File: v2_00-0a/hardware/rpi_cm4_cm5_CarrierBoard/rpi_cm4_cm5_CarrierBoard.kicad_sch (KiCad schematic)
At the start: 0 parts

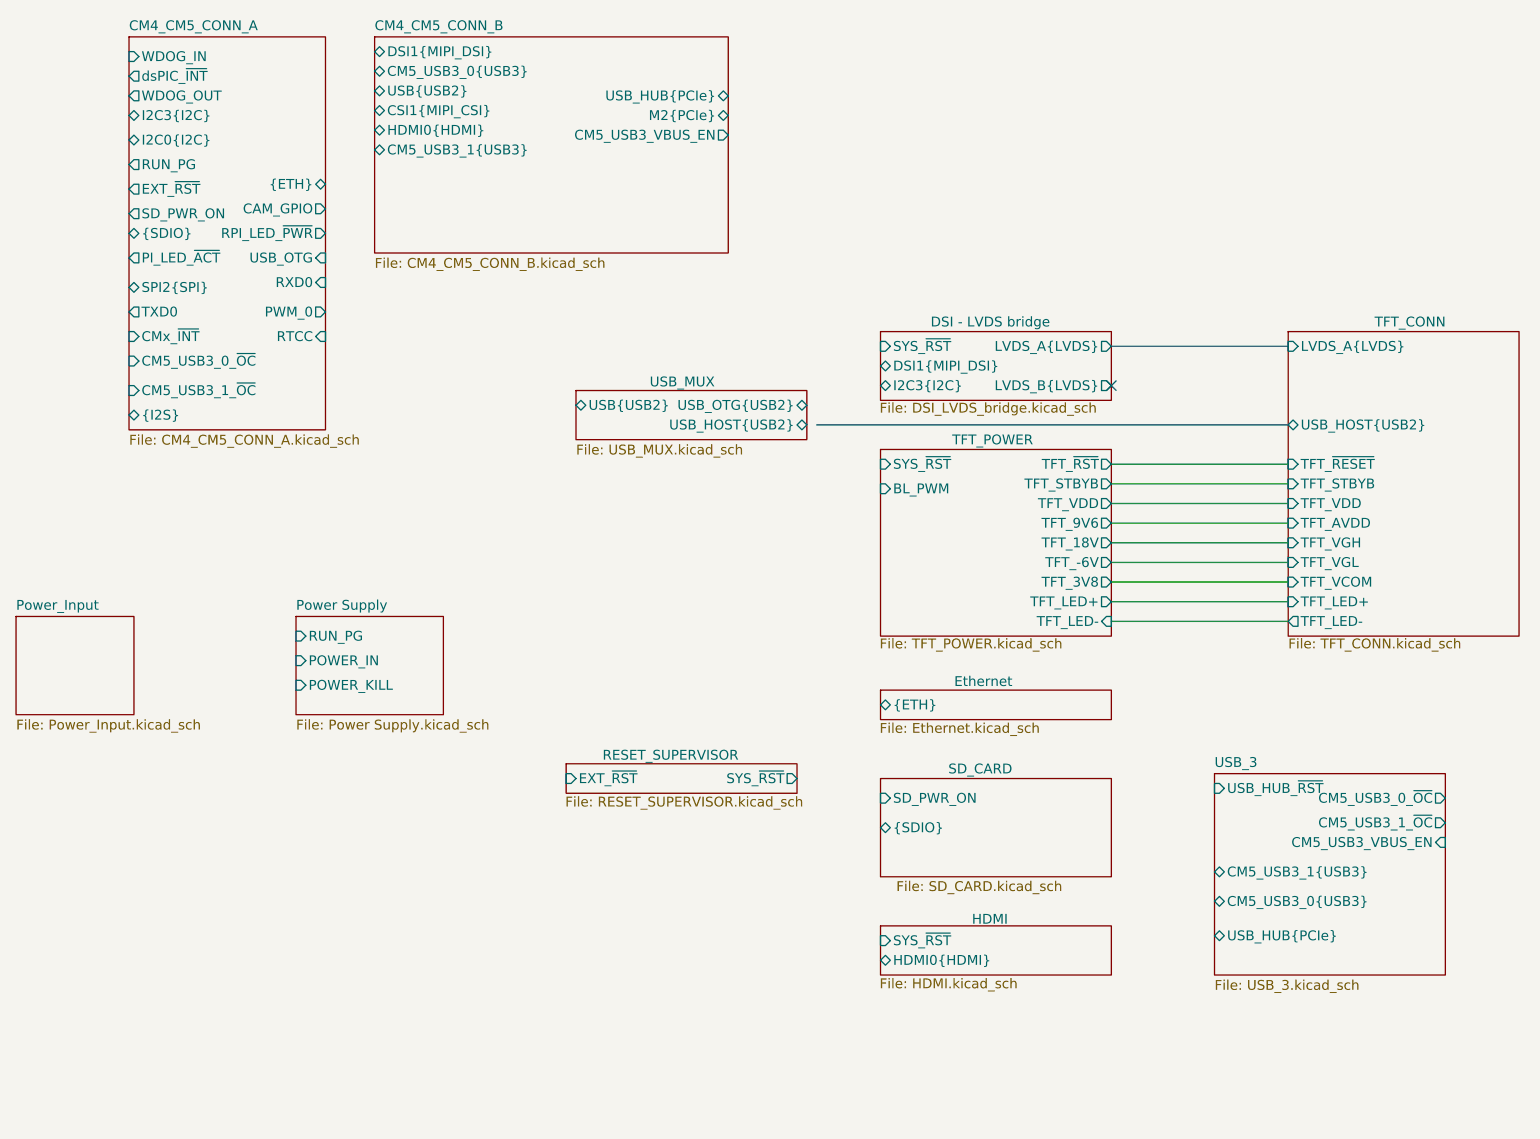
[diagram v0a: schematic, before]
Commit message: Add and modify existing schematics
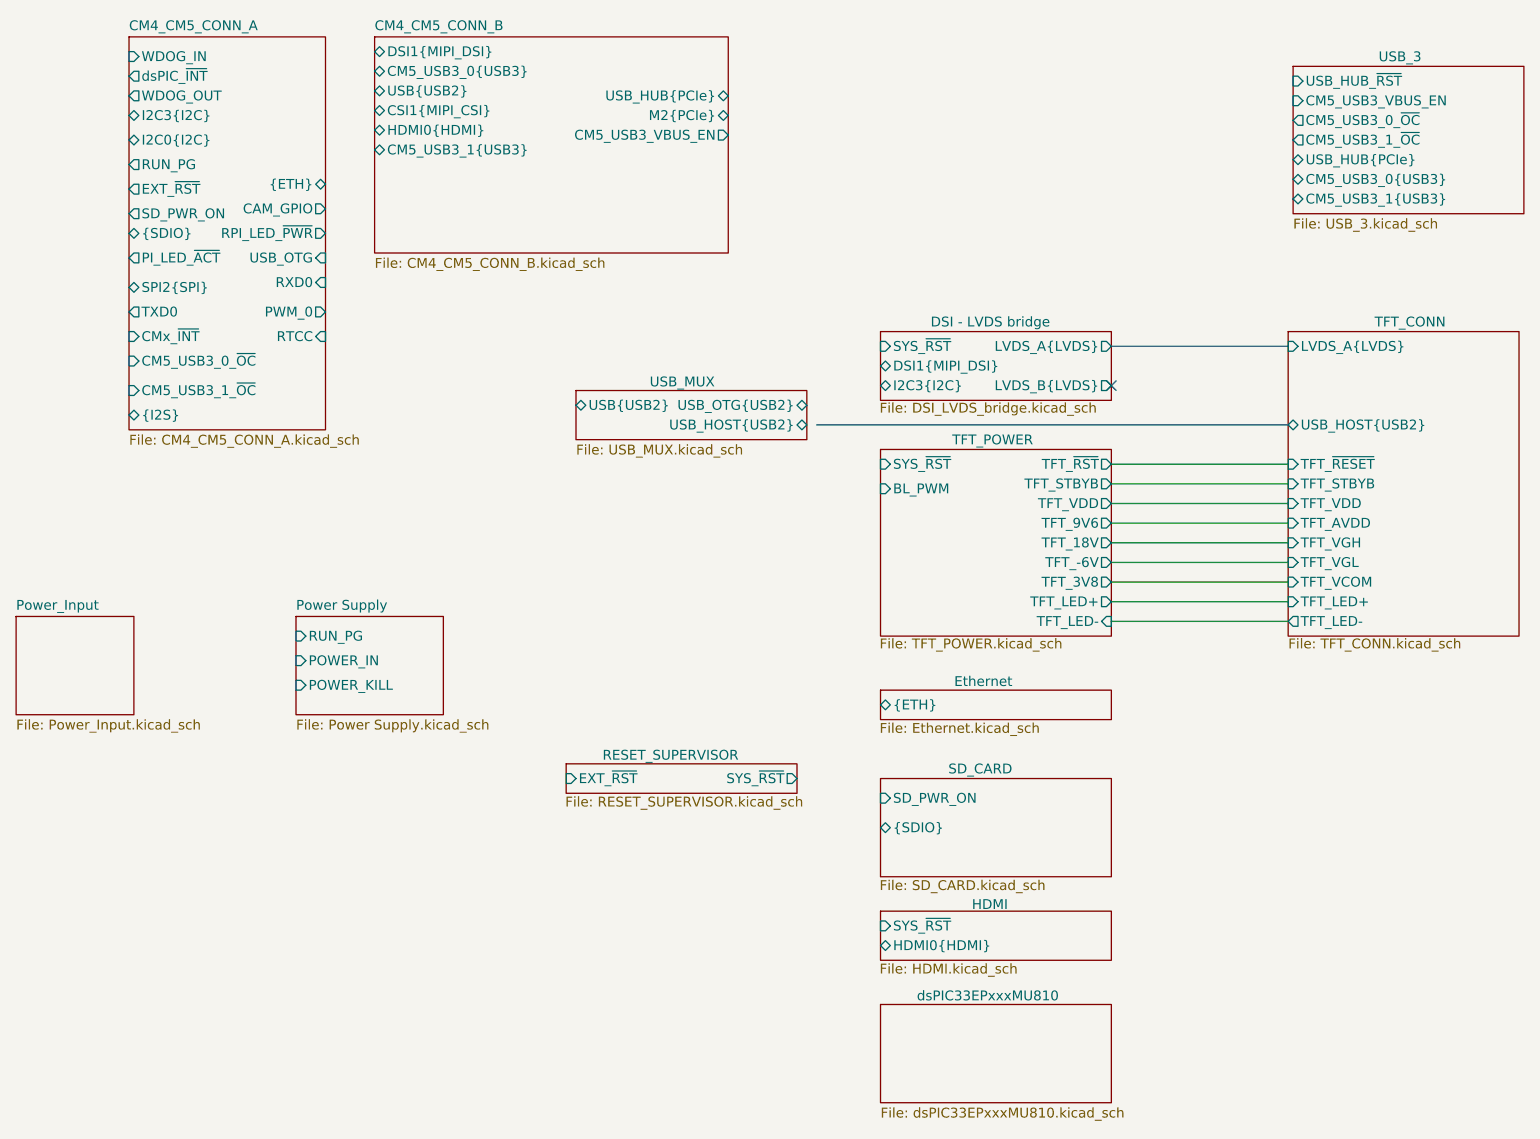
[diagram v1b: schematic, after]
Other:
- added sheet dsPIC33EPxxxMU810 (dsPIC33EPxxxMU810.kicad_sch)
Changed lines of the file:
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@@
 	)
 	(sheet
-		(at 241.935 120.65)
-		(size 29.845 26.035)
+		(at 252.095 29.21)
+		(size 29.845 19.05)
 		(exclude_from_sim no)
 		(in_bom yes)
 		(on_board yes)
 		(dnp no)
-		(fields_autoplaced yes)
 		(stroke
 			(width 0.1524)
@@
 		)
 		(property "Sheetname" "USB_3"
-			(at 241.935 119.9384 0)
+			(at 263.144 28.702 0)
 			(effects
 				(font
@@
 		)
 		(property "Sheetfile" "USB_3.kicad_sch"
-			(at 241.935 147.2696 0)
+			(at 252.095 48.8446 0)
 			(effects
 				(font
@@
 		)
 		(pin "USB_HUB_~{RST}" input
-			(at 241.935 122.555 180)
+			(at 252.095 31.115 180)
 			(effects
 				(font
@@
 		)
 		(pin "CM5_USB3_0{USB3}" bidirectional
-			(at 241.935 137.16 180)
+			(at 252.095 43.815 180)
 			(effects
 				(font
@@
 		)
 		(pin "CM5_USB3_1_~{OC}" output
-			(at 271.78 127 0)
-			(effects
-				(font
-					(size 1.27 1.27)
-				)
-				(justify right)
+			(at 252.095 38.735 180)
+			(effects
+				(font
+					(size 1.27 1.27)
+				)
+				(justify left)
 			)
 		)
 		(pin "CM5_USB3_0_~{OC}" output
-			(at 271.78 123.825 0)
-			(effects
-				(font
-					(size 1.27 1.27)
-				)
-				(justify right)
+			(at 252.095 36.195 180)
+			(effects
+				(font
+					(size 1.27 1.27)
+				)
+				(justify left)
 			)
 		)
 		(pin "CM5_USB3_VBUS_EN" input
-			(at 271.78 129.54 0)
-			(effects
-				(font
-					(size 1.27 1.27)
-				)
-				(justify right)
+			(at 252.095 33.655 180)
+			(effects
+				(font
+					(size 1.27 1.27)
+				)
+				(justify left)
 			)
 		)
 		(pin "CM5_USB3_1{USB3}" bidirectional
-			(at 241.935 133.35 180)
+			(at 252.095 46.355 180)
 			(effects
 				(font
@@
 		)
 		(pin "USB_HUB{PCIe}" bidirectional
-			(at 241.935 141.605 180)
+			(at 252.095 41.275 180)
 			(effects
 				(font
@@
 	)
 	(sheet
+		(at 198.755 150.495)
+		(size 29.845 12.7)
+		(exclude_from_sim no)
+		(in_bom yes)
+		(on_board yes)
+		(dnp no)
+		(stroke
+			(width 0.1524)
+			(type solid)
+		)
+		(fill
+			(color 0 0 0 0.0000)
+		)
+		(property "Sheetname" "dsPIC33EPxxxMU810"
+			(at 203.454 150.114 0)
+			(effects
+				(font
+					(size 1.27 1.27)
+				)
+				(justify left bottom)
+			)
+		)
+		(property "Sheetfile" "dsPIC33EPxxxMU810.kicad_sch"
+			(at 198.755 163.7796 0)
+			(effects
+				(font
+					(size 1.27 1.27)
+				)
+				(justify left top)
+			)
+		)
+		(instances
+			(project "rpi_cm4_cm5_CarrierBoard"
+				(path "/7dcdf741-90ca-4333-848c-806f4d64158e"
+					(page "15")
+				)
+			)
+		)
+	)
+	(sheet
 		(at 158.115 119.38)
 		(size 29.845 3.81)
@@
 		)
 		(property "Sheetfile" "SD_CARD.kicad_sch"
-			(at 200.787 134.493 0)
+			(at 198.628 134.366 0)
 			(effects
 				(font
@@
 	)
 	(sheet
-		(at 198.755 140.335)
+		(at 198.755 138.43)
 		(size 29.845 6.35)
 		(exclude_from_sim no)
@@
 		)
 		(property "Sheetname" "HDMI"
-			(at 210.566 140.208 0)
+			(at 210.566 138.303 0)
 			(effects
 				(font
@@
 		)
 		(property "Sheetfile" "HDMI.kicad_sch"
-			(at 198.628 147.066 0)
+			(at 198.628 145.161 0)
 			(effects
 				(font
@@
 		)
 		(pin "SYS_~{RST}" input
-			(at 198.755 142.24 180)
+			(at 198.755 140.335 180)
 			(effects
 				(font
@@
 		)
 		(pin "HDMI0{HDMI}" bidirectional
-			(at 198.755 144.78 180)
-			(effects
-				(font
+			(at 198.755 142.875 180)
+			(effects
+				(font
